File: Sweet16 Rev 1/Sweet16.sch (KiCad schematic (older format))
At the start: 72 parts, among them J1 Conn_01x09_Male, J10 SW_half_inverter, J11 R_clock, J12 OUT_clock, J13 SW_dual8_hex, J14 OUT_OUT, J15 R_sync_pitch_1, J16 SW_sync_1, J17 R_sync_pitch_2, J18 SW_sync_2, J19 Barrel_Jack, J2 Conn_01x09_Male, J20 R_sync_pitch_2, J21 SW_dual8_hex_2, J22 OUT_OUT, J23 OUT_CARRY_OUT, J3 Conn_01x09_Male, J4 Conn_01x09_Male, J5 OUT_OUT, J6 SW_run, J7 SW_BIN_DEC, J8 SW_UP_DN, J9 SW_clock_source, U1 40106, U2 4029, U3 4028, U4 4051, U5 4028, U6 4070, U7 4051, U8 TL072

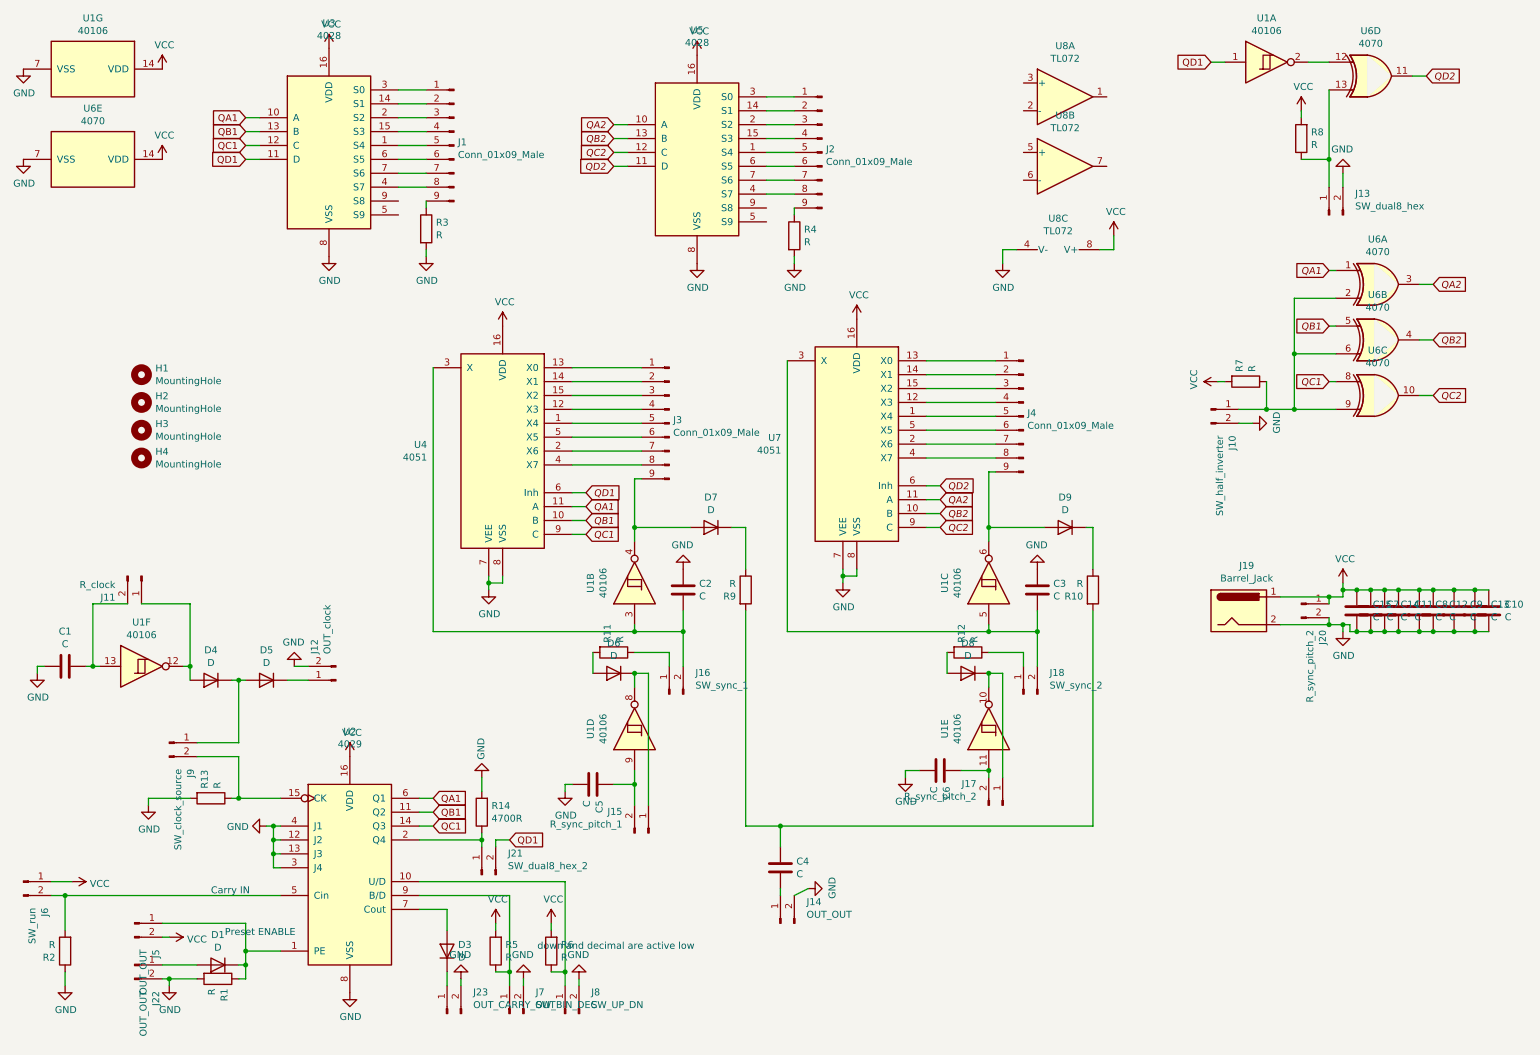
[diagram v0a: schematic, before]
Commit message: 48 wires to go
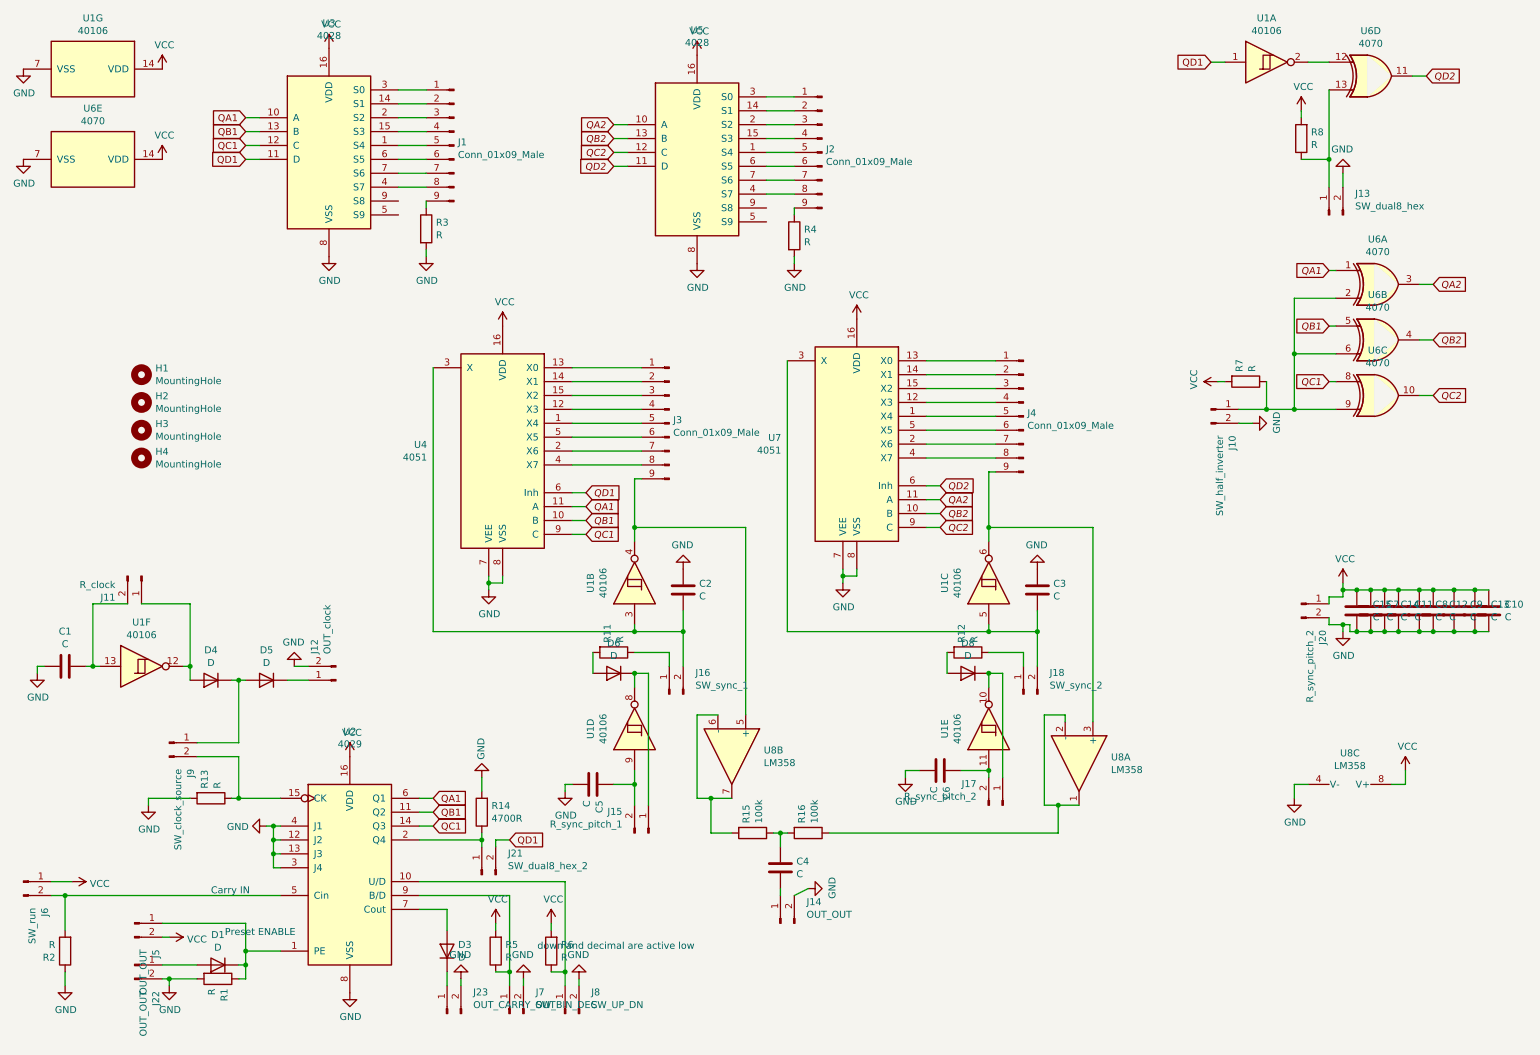
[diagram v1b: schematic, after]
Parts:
- removed D7, D9: D, Diode_THT:D_A-405_P7.62mm_Horizontal, symbol Device:D
- removed J19: Barrel_Jack, Connector_BarrelJack:BarrelJack_CUI_PJ-102AH_Horizontal, symbol Connector:Barrel_Jack
- removed R10, R9: R, Resistor_THT:R_Axial_DIN0207_L6.3mm_D2.5mm_P7.62mm_Horizontal, symbol Device:R
- removed U8: TL072, Package_DIP:DIP-8_W7.62mm_LongPads, symbol Amplifier_Operational:TL072
- added R15, R16: 100k, Resistor_THT:R_Axial_DIN0207_L6.3mm_D2.5mm_P7.62mm_Horizontal, symbol Device:R
- added U8: LM358, Package_DIP:DIP-8_W7.62mm_LongPads, symbol Amplifier_Operational:LM358
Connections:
- net GND: now also U8.4 (V-)
- net VCC: now also U8.8 (V+)
- net at J3.9 (Pin_9), U1.4: now also U8.5 (+)
- net at J4.9 (Pin_9), U1.6: now also U8.3 (+)
- net at C4.2: now also R15.1, R16.2
- new net: R16.1, U8.1, U8.2 (-)
- new net: R15.2, U8.6 (-), U8.7
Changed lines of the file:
@@
 	7550 4200 7550 4300
-$Comp
-L Device:R R9
-U 1 1 600316E2
-P 5800 4650
-F 0 "R9" H 5730 4604 50  0000 R CNN
-F 1 "R" H 5730 4695 50  0000 R CNN
-F 2 "Resistor_THT:R_Axial_DIN0207_L6.3mm_D2.5mm_P7.62mm_Horizontal" V 5730 4650 50  0001 C CNN
-F 3 "~" H 5800 4650 50  0001 C CNN
-	1    5800 4650
-	1    0    0    -1
-$EndComp
 $Comp
 L Connector:Conn_01x02_Male J10
@@
 	9550 3350 9750 3350
 $Comp
-L Device:R R10
-U 1 1 60329897
-P 8300 4650
-F 0 "R10" H 8230 4604 50  0000 R CNN
-F 1 "R" H 8230 4695 50  0000 R CNN
-F 2 "Resistor_THT:R_Axial_DIN0207_L6.3mm_D2.5mm_P7.62mm_Horizontal" V 8230 4650 50  0001 C CNN
-F 3 "~" H 8300 4650 50  0001 C CNN
-	1    8300 4650
-	1    0    0    -1
-$EndComp
-Wire Wire Line
-	5800 4800 5800 6350
-Wire Wire Line
-	8300 6350 8300 4800
-Wire Wire Line
-	5800 4200 5800 4500
-Wire Wire Line
-	8300 4200 8300 4500
-$Comp
 L Device:C C4
 U 1 1 603E27DA
@@
 $EndComp
 $Comp
-L Device:D D9
-U 1 1 5FD09EF1
-P 8100 4200
-F 0 "D9" H 8100 3983 50  0000 C CNN
-F 1 "D" H 8100 4074 50  0000 C CNN
-F 2 "Diode_THT:D_A-405_P7.62mm_Horizontal" H 8100 4200 50  0001 C CNN
-F 3 "~" H 8100 4200 50  0001 C CNN
-	1    8100 4200
-	-1   0    0    1
-$EndComp
-$Comp
-L Device:D D7
-U 1 1 5FD0D58A
-P 5550 4200
-F 0 "D7" H 5550 3983 50  0000 C CNN
-F 1 "D" H 5550 4074 50  0000 C CNN
-F 2 "Diode_THT:D_A-405_P7.62mm_Horizontal" H 5550 4200 50  0001 C CNN
-F 3 "~" H 5550 4200 50  0001 C CNN
-	1    5550 4200
-	-1   0    0    1
-$EndComp
-Wire Wire Line
-	5700 4200 5800 4200
-Wire Wire Line
-	8300 4200 8250 4200
-$Comp
 L Device:D D6
 U 1 1 5FD3EE69
@@
 	-1   0    0    1
 $EndComp
-Wire Wire Line
-	6050 6350 8300 6350
-Connection ~ 6050 6350
-Wire Wire Line
-	6050 6350 6050 6500
-Wire Wire Line
-	5800 6350 6050 6350
 $Comp
 L Connector:Conn_01x02_Male J14
@@
 $EndComp
 $Comp
-L Connector:Barrel_Jack J19
-U 1 1 600C4E4A
-P 9350 4800
-F 0 "J19" H 9407 5125 50  0000 C CNN
-F 1 "Barrel_Jack" H 9407 5034 50  0000 C CNN
-F 2 "Connector_BarrelJack:BarrelJack_CUI_PJ-102AH_Horizontal" H 9400 4760 50  0001 C CNN
-F 3 "~" H 9400 4760 50  0001 C CNN
-	1    9350 4800
-	1    0    0    -1
-$EndComp
-$Comp
 L Connector:Conn_01x02_Male J20
 U 1 1 600C58B1
@@
 $EndComp
 Wire Wire Line
-	9650 4700 10000 4700
-Wire Wire Line
 	10100 4700 10100 4650
 Wire Wire Line
@@
 	10100 4650 10100 4600
 Wire Wire Line
-	9650 4900 10000 4900
-Wire Wire Line
 	10100 4900 10100 4950
 Wire Wire Line
@@
 Wire Wire Line
 	10000 4850 10000 4900
-Connection ~ 10000 4900
 Wire Wire Line
 	10000 4900 10100 4900
 Wire Wire Line
 	10000 4750 10000 4700
-Connection ~ 10000 4700
 Wire Wire Line
 	10000 4700 10100 4700
@@
 Wire Wire Line
 	10400 4650 10500 4650
-Wire Wire Line
-	5000 4200 5400 4200
 $Comp
 L power:GND #PWR0138
@@
 	-1   0    0    1
 $EndComp
-Wire Wire Line
-	7550 4200 7950 4200
 $Comp
 L power:GND #PWR0139
@@
 	1600 7050 2200 7050
 $Comp
-L Amplifier_Operational:TL072 U8
-U 1 1 61535B29
-P 8100 1100
-F 0 "U8" H 8100 1467 50  0000 C CNN
-F 1 "TL072" H 8100 1376 50  0000 C CNN
-F 2 "Package_DIP:DIP-8_W7.62mm_LongPads" H 8100 1100 50  0001 C CNN
-F 3 "http://www.ti.com/lit/ds/symlink/tl071.pdf" H 8100 1100 50  0001 C CNN
-	1    8100 1100
-	1    0    0    -1
-$EndComp
-$Comp
-L Amplifier_Operational:TL072 U8
-U 2 1 61536DC3
-P 8100 1600
-F 0 "U8" H 8100 1967 50  0000 C CNN
-F 1 "TL072" H 8100 1876 50  0000 C CNN
-F 2 "Package_DIP:DIP-8_W7.62mm_LongPads" H 8100 1600 50  0001 C CNN
-F 3 "http://www.ti.com/lit/ds/symlink/tl071.pdf" H 8100 1600 50  0001 C CNN
-	2    8100 1600
-	1    0    0    -1
-$EndComp
-$Comp
-L Amplifier_Operational:TL072 U8
-U 3 1 6153A199
-P 8050 2300
-F 0 "U8" V 7725 2300 50  0000 C CNN
-F 1 "TL072" V 7816 2300 50  0000 C CNN
-F 2 "Package_DIP:DIP-8_W7.62mm_LongPads" H 8050 2300 50  0001 C CNN
-F 3 "http://www.ti.com/lit/ds/symlink/tl071.pdf" H 8050 2300 50  0001 C CNN
-	3    8050 2300
-	0    1    1    0
-$EndComp
-$Comp
 L Device:C C15
 U 1 1 6153CD4F
@@
 L power:GND #PWR0142
 U 1 1 6154B30B
-P 7650 2300
-F 0 "#PWR0142" H 7650 2050 50  0001 C CNN
-F 1 "GND" H 7655 2127 50  0000 C CNN
-F 2 "" H 7650 2300 50  0001 C CNN
-F 3 "" H 7650 2300 50  0001 C CNN
-	1    7650 2300
+P 9750 6150
+F 0 "#PWR0142" H 9750 5900 50  0001 C CNN
+F 1 "GND" H 9755 5977 50  0000 C CNN
+F 2 "" H 9750 6150 50  0001 C CNN
+F 3 "" H 9750 6150 50  0001 C CNN
+	1    9750 6150
 	1    0    0    -1
 $EndComp
@@
 L power:VCC #PWR0143
 U 1 1 6154BF9B
-P 8450 2100
-F 0 "#PWR0143" H 8450 1950 50  0001 C CNN
-F 1 "VCC" H 8465 2273 50  0000 C CNN
-F 2 "" H 8450 2100 50  0001 C CNN
-F 3 "" H 8450 2100 50  0001 C CNN
-	1    8450 2100
-	1    0    0    -1
-$EndComp
-Wire Wire Line
-	8350 2200 8450 2200
-Wire Wire Line
-	8450 2200 8450 2100
-Wire Wire Line
-	7750 2200 7650 2200
-Wire Wire Line
-	7650 2200 7650 2300
+P 10550 5950
+F 0 "#PWR0143" H 10550 5800 50  0001 C CNN
+F 1 "VCC" H 10565 6123 50  0000 C CNN
+F 2 "" H 10550 5950 50  0001 C CNN
+F 3 "" H 10550 5950 50  0001 C CNN
+	1    10550 5950
+	1    0    0    -1
+$EndComp
+Wire Wire Line
+	10450 6050 10550 6050
+Wire Wire Line
+	10550 6050 10550 5950
+Wire Wire Line
+	9850 6050 9750 6050
+Wire Wire Line
+	9750 6050 9750 6150
+Wire Wire Line
+	5600 5550 5450 5550
+Wire Wire Line
+	5450 5550 5450 6150
+Wire Wire Line
+	5450 6150 5550 6150
+Wire Wire Line
+	8100 5550 8100 5600
+Wire Wire Line
+	8100 5550 7950 5550
+Wire Wire Line
+	7950 5550 7950 6200
+Wire Wire Line
+	7950 6200 8050 6200
+$Comp
+L Amplifier_Operational:LM358 U8
+U 1 1 6112DB96
+P 8200 5900
+F 0 "U8" V 8154 6130 50  0000 L CNN
+F 1 "LM358" V 8245 6130 50  0000 L CNN
+F 2 "Package_DIP:DIP-8_W7.62mm_LongPads" H 8200 5900 50  0001 C CNN
+F 3 "http://www.ti.com/lit/ds/symlink/lm2904-n.pdf" H 8200 5900 50  0001 C CNN
+	1    8200 5900
+	0    1    1    0
+$EndComp
+$Comp
+L Amplifier_Operational:LM358 U8
+U 2 1 61132740
+P 5700 5850
+F 0 "U8" V 5654 6080 50  0000 L CNN
+F 1 "LM358" V 5745 6080 50  0000 L CNN
+F 2 "Package_DIP:DIP-8_W7.62mm_LongPads" H 5700 5850 50  0001 C CNN
+F 3 "http://www.ti.com/lit/ds/symlink/lm2904-n.pdf" H 5700 5850 50  0001 C CNN
+	2    5700 5850
+	0    1    1    0
+$EndComp
+$Comp
+L Amplifier_Operational:LM358 U8
+U 3 1 61137CD1
+P 10150 6150
+F 0 "U8" V 9825 6150 50  0000 C CNN
+F 1 "LM358" V 9916 6150 50  0000 C CNN
+F 2 "Package_DIP:DIP-8_W7.62mm_LongPads" H 10150 6150 50  0001 C CNN
+F 3 "http://www.ti.com/lit/ds/symlink/lm2904-n.pdf" H 10150 6150 50  0001 C CNN
+	3    10150 6150
+	0    1    1    0
+$EndComp
+$Comp
+L Device:R R15
+U 1 1 6120315D
+P 5850 6400
+F 0 "R15" H 5780 6354 50  0000 R CNN
+F 1 "100k" H 5780 6445 50  0000 R CNN
+F 2 "Resistor_THT:R_Axial_DIN0207_L6.3mm_D2.5mm_P7.62mm_Horizontal" V 5780 6400 50  0001 C CNN
+F 3 "~" H 5850 6400 50  0001 C CNN
+	1    5850 6400
+	0    1    1    0
+$EndComp
+$Comp
+L Device:R R16
+U 1 1 61203A58
+P 6250 6400
+F 0 "R16" H 6180 6354 50  0000 R CNN
+F 1 "100k" H 6180 6445 50  0000 R CNN
+F 2 "Resistor_THT:R_Axial_DIN0207_L6.3mm_D2.5mm_P7.62mm_Horizontal" V 6180 6400 50  0001 C CNN
+F 3 "~" H 6250 6400 50  0001 C CNN
+	1    6250 6400
+	0    1    1    0
+$EndComp
+Wire Wire Line
+	5550 6150 5550 6400
+Wire Wire Line
+	5550 6400 5700 6400
+Connection ~ 5550 6150
+Wire Wire Line
+	5550 6150 5700 6150
+Wire Wire Line
+	6000 6400 6050 6400
+Wire Wire Line
+	6050 6400 6050 6500
+Wire Wire Line
+	6100 6400 6050 6400
+Connection ~ 6050 6400
+Wire Wire Line
+	6400 6400 8050 6400
+Wire Wire Line
+	8050 6400 8050 6200
+Connection ~ 8050 6200
+Wire Wire Line
+	8050 6200 8200 6200
+Wire Wire Line
+	7550 4200 8300 4200
+Wire Wire Line
+	8300 4200 8300 5600
+Wire Wire Line
+	5000 4200 5800 4200
+Wire Wire Line
+	5800 4200 5800 5550
 $EndSCHEMATC
